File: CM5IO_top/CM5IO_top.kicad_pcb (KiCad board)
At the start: 2 copper layers, 59.7 x 56.3 mm, 55 parts, among them J1 USB_C_Receptacle_USB2.0, J10 J_DShot600_FC, J3 J_PSU_EN, J4 J_ESP_DBG_UART, J7 J_FC_UART, J8 THD-20-R, J9 J_DShot600_ESC, Q1 AO3401A, Q2 Q_NPN_BEC, Q3 Q_NPN_BEC, Q4 AO3401A, SW1 SW_RESET, SW2 SW_BOOT, SW3 FORCE_PWR, U1 ESP32-S3-WROOM-1, U2 Wio-SX1262, U3 AP7361C-33E, U4 AP7361C-33E

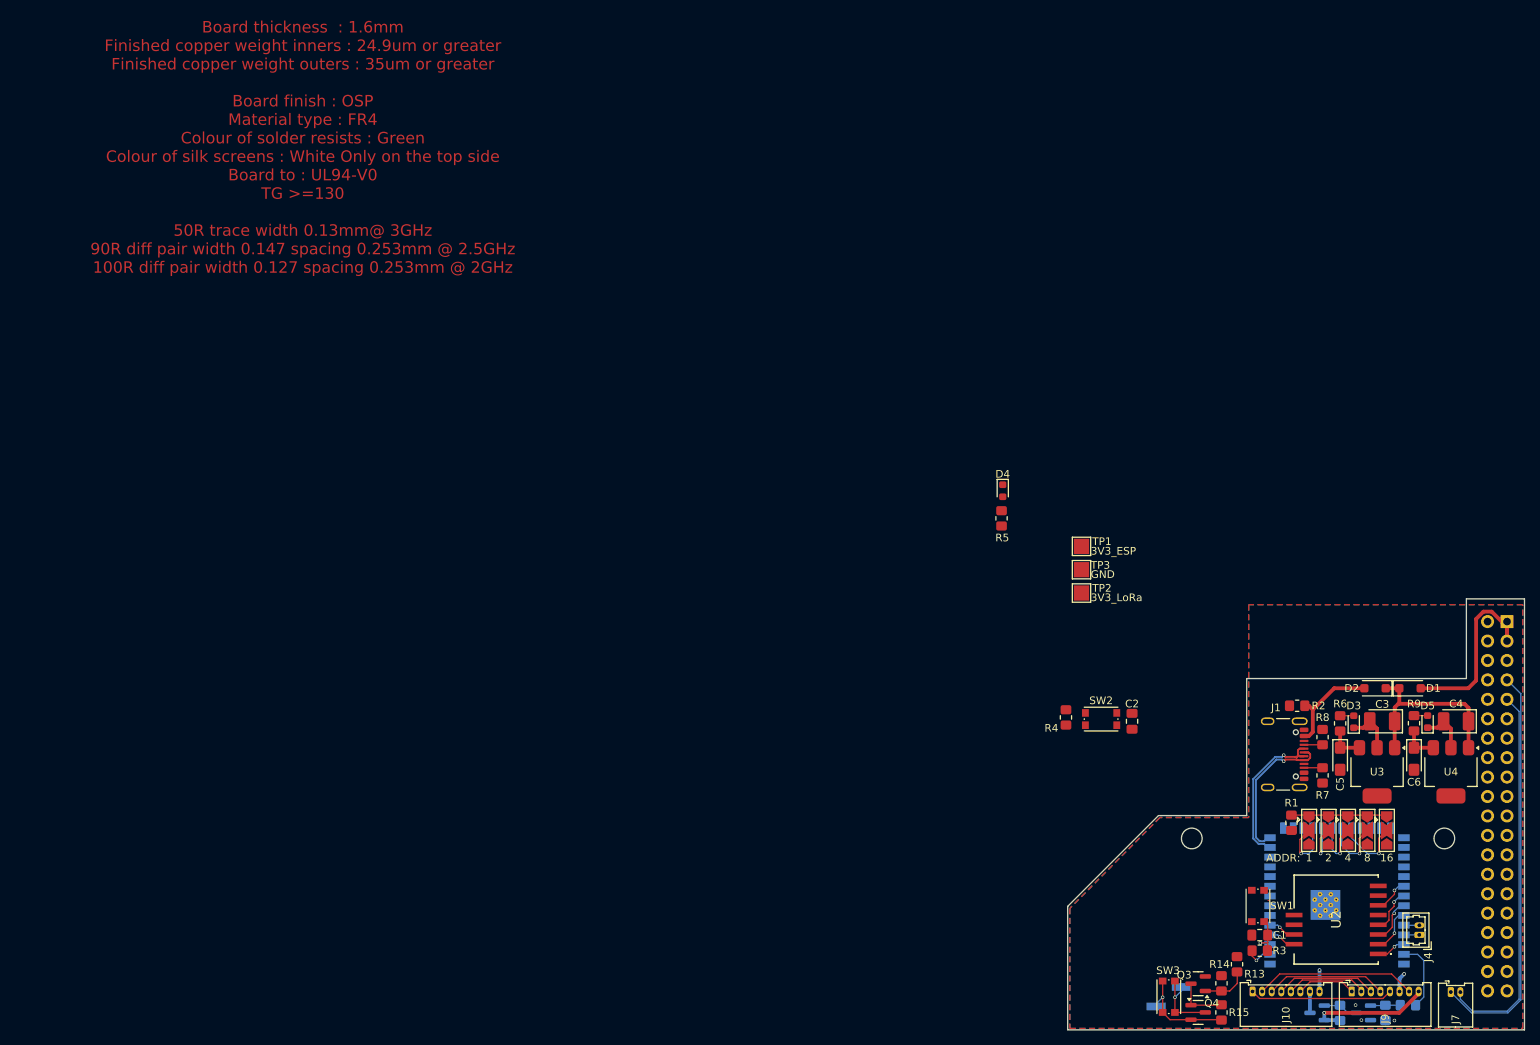
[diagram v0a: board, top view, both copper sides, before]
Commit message: upper board finished (I hope)
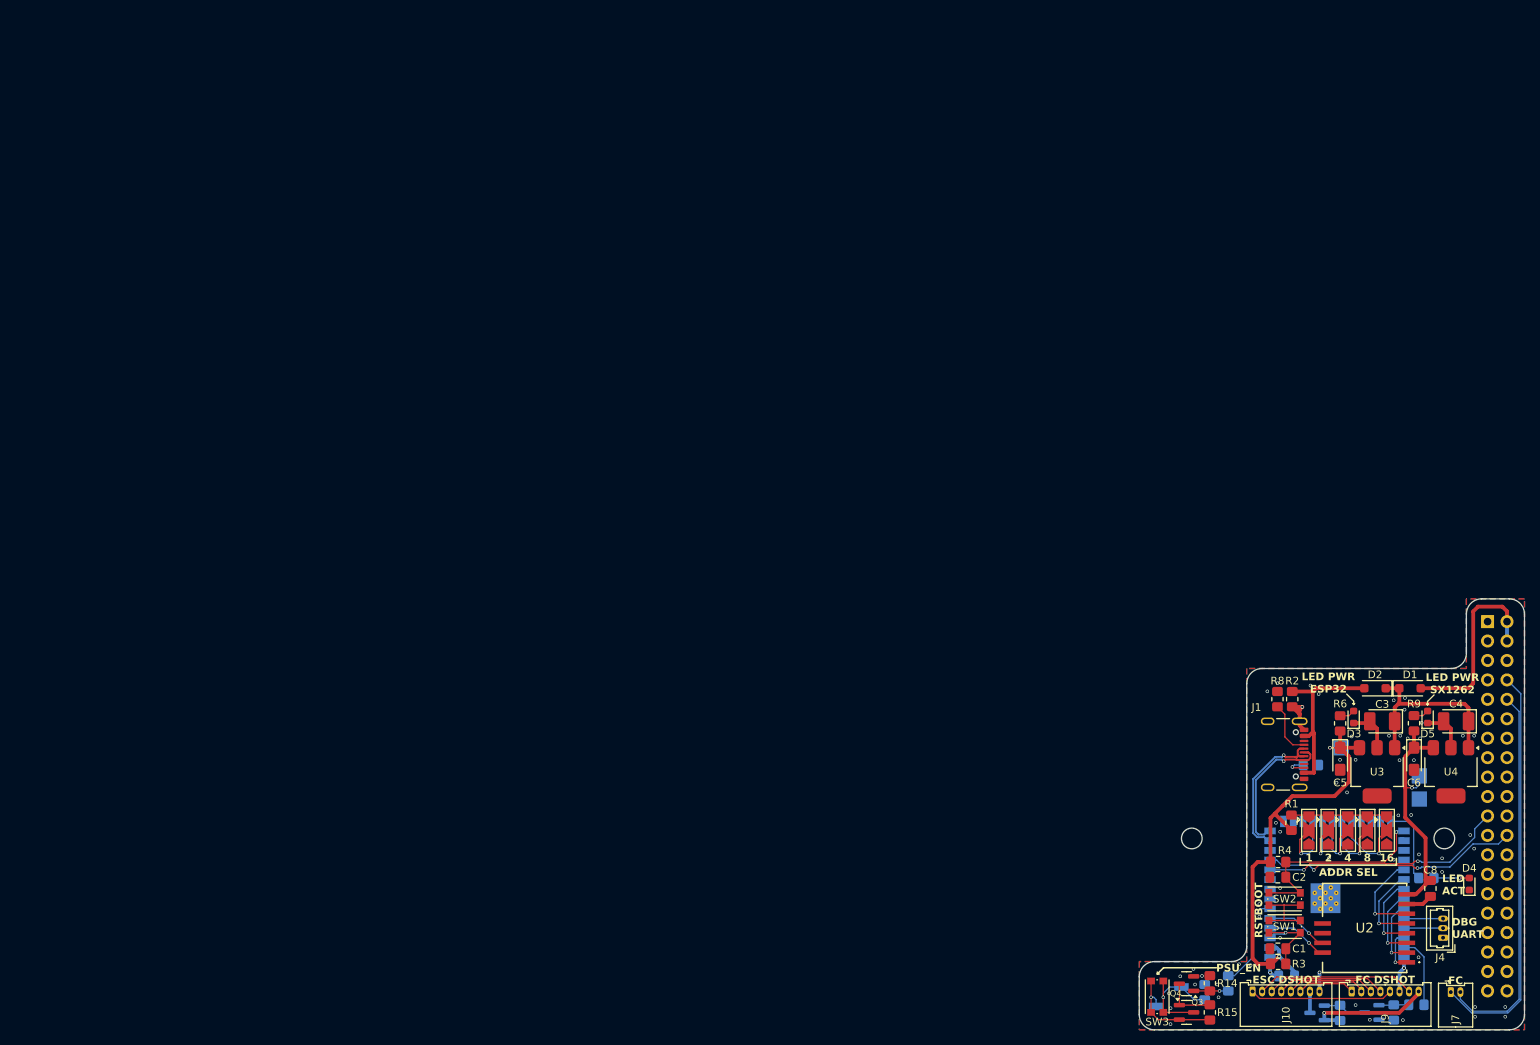
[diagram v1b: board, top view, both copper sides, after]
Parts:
- added C7: 470nF, Capacitor_SMD:C_0805_2012Metric_Pad1.18x1.45mm_HandSolder, B.Cu at (174.9, 139.5)
- added C8: 470nF, Capacitor_SMD:C_0805_2012Metric_Pad1.18x1.45mm_HandSolder, F.Cu at (193.7, 128.0)
- added R16: 10K, Resistor_SMD:R_0805_2012Metric_Pad1.20x1.40mm_HandSolder, B.Cu at (164.2, 141.6)
- C3, C4: value 4.7uF 25v -> 4.7uF 35v
- C5, C6: value 4.7uF 6.3v -> 4.7uF 10v
- J3: footprint Connector_PinHeader_2.54mm:PinHeader_1x02_P2.54mm_Vertical_SMD_Pin1Left -> Connector_PinSocket_2.54mm:PinSocket_1x02_P2.54mm_Vertical_SMD_Pin1Left
- J4: footprint Connector_Molex:Molex_PicoBlade_53047-0210_1x02_P1.25mm_Vertical -> Connector_Molex:Molex_PicoBlade_53047-0310_1x03_P1.25mm_Vertical
- J8: footprint Connector_PinHeader_2.54mm:PinHeader_2x20_P2.54mm_Vertical -> Connector_PinSocket_2.54mm:PinSocket_2x20_P2.54mm_Vertical
- R13, R5, R7, TP1, TP2, TP3: moved to B.Cu
- moved D4 79.7 mm to (198.8, 127.5), turned to 90 degrees
- moved R5 72.7 mm to (193.1, 126.7), turned to 0 degrees
- moved TP3 53.4 mm to (192.2, 116.4), turned to 180 degrees
- moved TP2 50.2 mm to (192.2, 113.3), turned to 180 degrees
- moved TP1 42.9 mm to (182.0, 109.6), turned to 180 degrees
- moved SW2 33.6 mm to (174.6, 129.4), turned to 180 degrees
- moved R4 33.6 mm to (173.8, 124.6), turned to 0 degrees
- moved C2 27.9 mm to (173.7, 126.6), turned to 0 degrees
- moved R8 7.70 mm to (173.7, 103.3)
- moved SW1 4.41 mm to (174.6, 133.0), turned to 0 degrees
- moved U2 3.88 mm to (185.1, 133.2)
- moved J4 3.12 mm to (195.3, 134.5)
- moved R3 2.96 mm to (173.8, 137.9)
- moved C1 2.96 mm to (173.7, 135.9)
- moved R13 2.74 mm to (167.3, 140.4)
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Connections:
- J4 pad 1: Net-(J4-Pin_1) -> GND
- J8 pad 1: /+5v_RPi -> unconnected-(J8-Pin_1-Pad1)
- J8 pad 10: GND -> /GPIO15_UART_RX
- J8 pad 11: /GPIO18 -> /GPIO17
- J8 pad 12: /GPIO17 -> /GPIO18
- J8 pad 13: GND -> /GPIO27
- J8 pad 14: /GPIO27 -> GND
- J8 pad 15: /GPIO23 -> /GPIO22
- J8 pad 16: /GPIO22 -> /GPIO23
- J8 pad 17: /GPIO24 -> unconnected-(J8-Pin_17-Pad17)
- J8 pad 18: unconnected-(J8-Pin_18-Pad18) -> /GPIO24
- J8 pad 19: GND -> /GPIO10
- J8 pad 2: unconnected-(J8-Pin_2-Pad2) -> /+5v_RPi
- J8 pad 20: /GPIO10 -> GND
- J8 pad 21: /GPIO25 -> /GPIO9
- J8 pad 22: /GPIO9 -> /GPIO25
- J8 pad 23: /GPIO8 -> /GPIO11
- J8 pad 24: /GPIO11 -> /GPIO8
- J8 pad 25: /GPIO7 -> GND
- J8 pad 26: GND -> /GPIO7
- J8 pad 29: GND -> /GPIO5
- J8 pad 3: /+5v_RPi -> /GPIO2
- J8 pad 30: /GPIO5 -> GND
- J8 pad 31: /GPIO12 -> /GPIO6
- J8 pad 32: /GPIO6 -> /GPIO12
- J8 pad 33: GND -> /GPIO13
- J8 pad 34: /GPIO13 -> GND
- J8 pad 35: /GPIO16 -> /GPIO19
- J8 pad 36: /GPIO19 -> /GPIO16
- J8 pad 37: /GPIO20 -> /GPIO26
- J8 pad 38: /GPIO26 -> /GPIO20
- J8 pad 39: /GPIO21 -> GND
- J8 pad 4: /GPIO2 -> /+5v_RPi
- J8 pad 40: GND -> /GPIO21
- J8 pad 5: GND -> /GPIO3
- J8 pad 6: /GPIO3 -> GND
- J8 pad 7: /GPIO14_UART_TX -> /GPIO4
- J8 pad 8: /GPIO4 -> /GPIO14_UART_TX
- J8 pad 9: /GPIO15_UART_RX -> GND
- U1 pad 16: /Comm/LED_ACT -> unconnected-(U1-IO46-Pad16)
- U1 pad 26: unconnected-(U1-IO45-Pad26) -> /Comm/LED_ACT
- U1 pad 31: unconnected-(U1-IO38-Pad31) -> /Comm/LORA_SPI_CS
- U1 pad 32: /Comm/LORA_SPI_CS -> /Comm/LORA_RESET
- U1 pad 36: Net-(J4-Pin_2) -> Net-(J4-Pin_3)
- U1 pad 37: Net-(J4-Pin_1) -> Net-(J4-Pin_2)
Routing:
- net /+3.3v_ESP: track 8.31 -> 57.7 mm, vias 1 -> 2
- net /GPIO8: track 0.00 -> 33.7 mm, vias 0 -> 2
- net /GPIO9: track 0.00 -> 32.1 mm, vias 0 -> 2
- net /Comm/BOOT_MODE: track 0.00 -> 27.4 mm, vias 0 -> 1
- net /+3.3v_LoRa: track 4.73 -> 31.0 mm, vias 0 -> 1
- net GND: track 18.4 -> 44.0 mm, vias 5 -> 60
- net /Comm/KILLSWITCH_PSU_CTL: track 0.00 -> 12.2 mm
- net /Comm/LORA_RESET: track 0.00 -> 11.0 mm, vias 0 -> 1
- net /Comm/LED_ACT: track 0.00 -> 10.2 mm
- net /+5v_USB: track 13.4 -> 22.9 mm
- net /Comm/LORA_SPI_CS: track 4.68 -> 12.0 mm
- net /PSU_CTL_EN: track 9.77 -> 15.0 mm
- net Net-(J4-Pin_3): track 0.00 -> 5.12 mm
- net /Comm/ENABLE: track 6.40 -> 11.3 mm
- net Net-(J1-CC1): track 2.42 -> 7.27 mm
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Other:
- board size 59.7 x 56.3 mm -> 50.3 x 56.3 mm
- board text added: "39"
- board text added: "40"
- board text added: "ADDR SEL"
- board text added: "BOOT"
- board text added: "CM5IO drone board IARC Hat"
- board text added: "DBG UART"
- board text added: "ESC DSHOT"
- board text added: "FC"
- board text added: "FC DSHOT"
- board text added: "LED ACT"
- board text added: "LED PWR ESP32"
- board text added: "LED PWR SX1262"
- board text added: "PSU_EN"
- board text added: "RST"
- board text added: "Solder 10K to disable PSU autostart"
- board text added: "rev. 1.0, 01.2026"
- board text removed: "ADDR:"
- board text removed: "Board thickness : 1.6mm Finished copper weight inners : 24.9um or greater Finished copper weight outers : 35um or greater Board finish : OSP Material type : FR4 Colour of solder resists : Green Colour of silk screens : White Only on the top side Board to : UL94-V0 TG >=130 50R trace width 0.13mm@ 3GHz 90R diff pair width 0.147 spacing 0.253mm @ 2.5GHz 100R diff pair width 0.127 spacing 0.253mm @ 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"
